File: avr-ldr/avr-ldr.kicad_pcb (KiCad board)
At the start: 2 copper layers, 54.6 x 35.6 mm, 26 parts, among them CON1 AVR-ISP-6, IC1 ATTINY2313-P, P1 RJ11, P2 CONN_01X05, U1 PCA82C250, Y1 4MHz

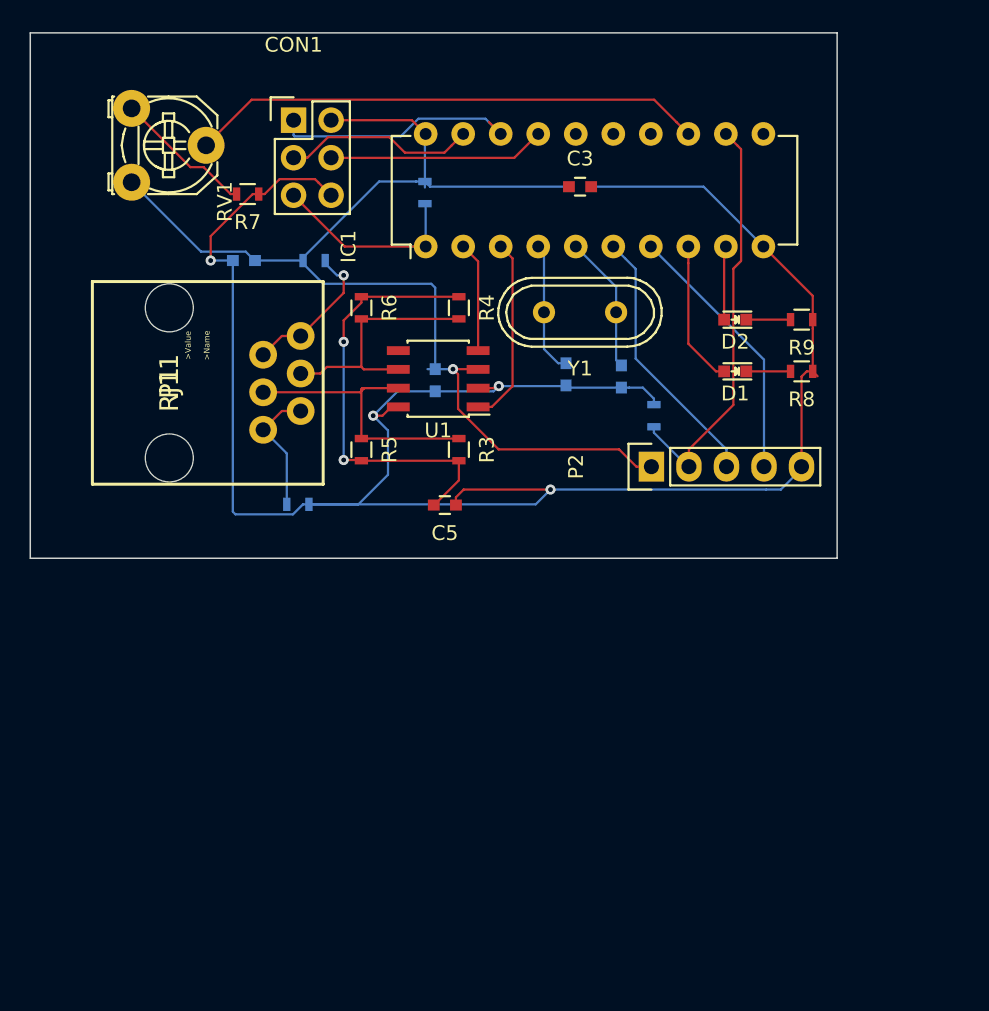
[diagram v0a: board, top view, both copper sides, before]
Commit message: Attempt #2 at my PCB design
Guess I may actually create this one?!
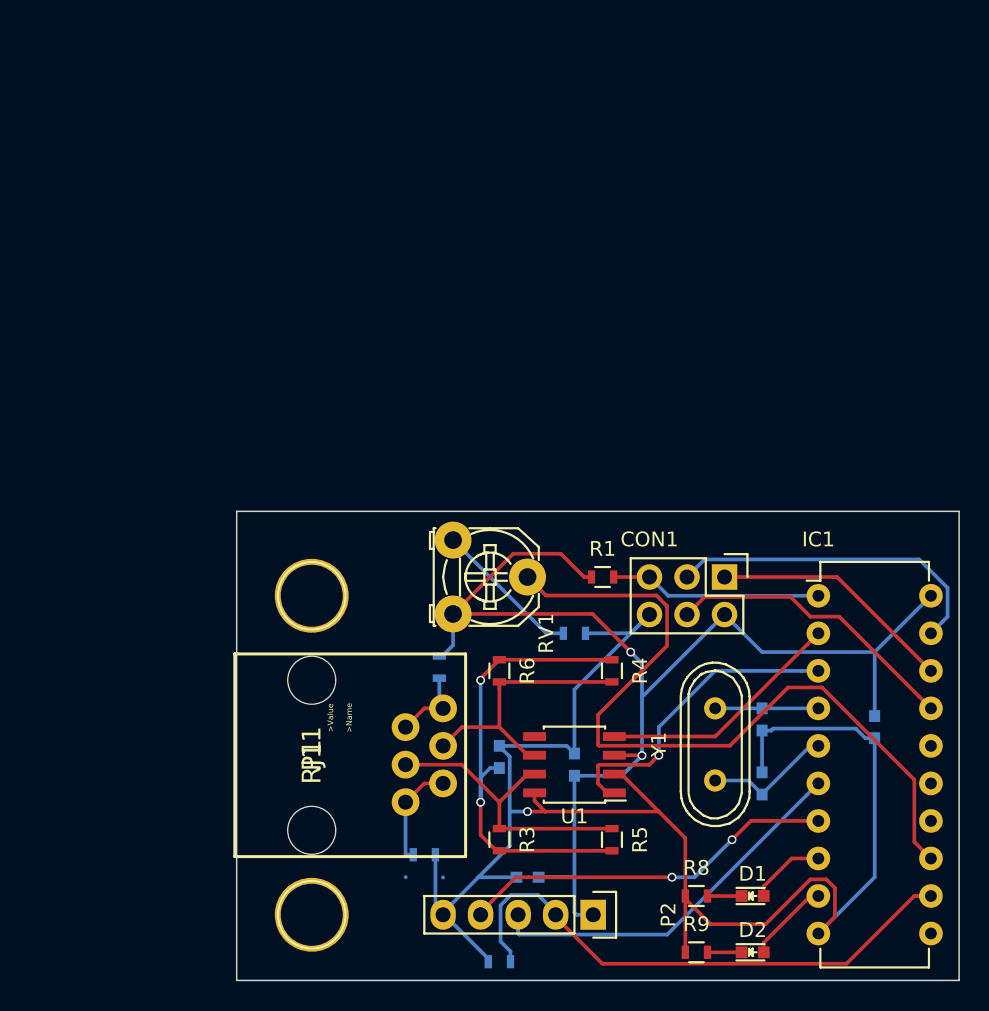
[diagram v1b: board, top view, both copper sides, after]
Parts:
- added REF**: 1pin, Connect:1pin, F.Cu at (116.8, 144.8)
- added REF**: 1pin, Connect:1pin, F.Cu at (116.8, 123.2)
- C3, C5, R7: moved to B.Cu
- R1: moved to F.Cu
- moved C6 45.9 mm to (131.4, 142.2)
- moved R9 43.4 mm to (142.9, 147.3), turned to 0 degrees
- moved D2 42.8 mm to (146.7, 147.3), turned to 0 degrees
- moved CON1 42.5 mm to (144.8, 121.9), turned to 270 degrees
- moved C3 41.7 mm to (154.9, 132.1), turned to 270 degrees
- moved R2 38.4 mm to (129.5, 148.0), turned to 0 degrees
- moved R7 37.1 mm to (134.6, 125.7)
- moved RV1 36.4 mm to (126.4, 119.4)
- moved R8 36.2 mm to (142.9, 143.5), turned to 0 degrees
- moved IC1 35.6 mm to (151.1, 123.2), turned to 0 degrees
- moved D1 35.5 mm to (146.7, 143.5), turned to 0 degrees
- moved R5 31.4 mm to (137.2, 139.7)
- moved Y1 30.6 mm to (144.1, 133.3), turned to 90 degrees
- moved P2 30.6 mm to (135.9, 144.8), turned to 270 degrees
- moved C2 29.1 mm to (147.3, 135.9), turned to 90 degrees
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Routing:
- net GND: track 142.8 -> 114.4 mm, vias 4 -> 1
- net Net-(IC1-Pad13): track 34.9 -> 53.0 mm
- net LDR_OUT: track 28.1 -> 37.7 mm
- net SCK: track 13.0 -> 22.5 mm
- net AVR_RXD: track 7.46 -> 16.7 mm
- net AVR_TXD: track 13.2 -> 21.3 mm, vias 0 -> 1
- net INPUT_A: track 18.1 -> 25.9 mm
- net INPUT_B: track 18.1 -> 25.7 mm, vias 0 -> 2
- net Net-(P1-Pad1): track 10.8 -> 5.22 mm, vias 1 -> 0
- net MOSI: track 14.7 -> 20.1 mm
- net Net-(D1-Pad2): track 9.78 -> 5.13 mm
- net VCC: track 81.0 -> 84.8 mm, vias 1 -> 2
- net Net-(C5-Pad2): track 29.9 -> 32.5 mm
- net Net-(C1-Pad1): track 8.99 -> 6.98 mm
- net Net-(P1-Pad5): track 8.77 -> 7.16 mm
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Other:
- board size 54.6 x 35.6 mm -> 48.9 x 31.8 mm
- net class Default: clearance 0.1524 -> 0.2; trace_width 0.1524 -> 0.25; via_dia 0.6858 -> 0.6; via_drill 0.3302 -> 0.4
- rule trace_clearance: 0.1524 -> 0.2
- rule trace_min: 0.1524 -> 0.2
- rule via_min_drill: 0.3302 -> 0.3
- rule via_min_size: 0.6858 -> 0.4
- board text added: "V2016.04.23"
